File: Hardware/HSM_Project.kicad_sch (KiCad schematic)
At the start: 0 parts

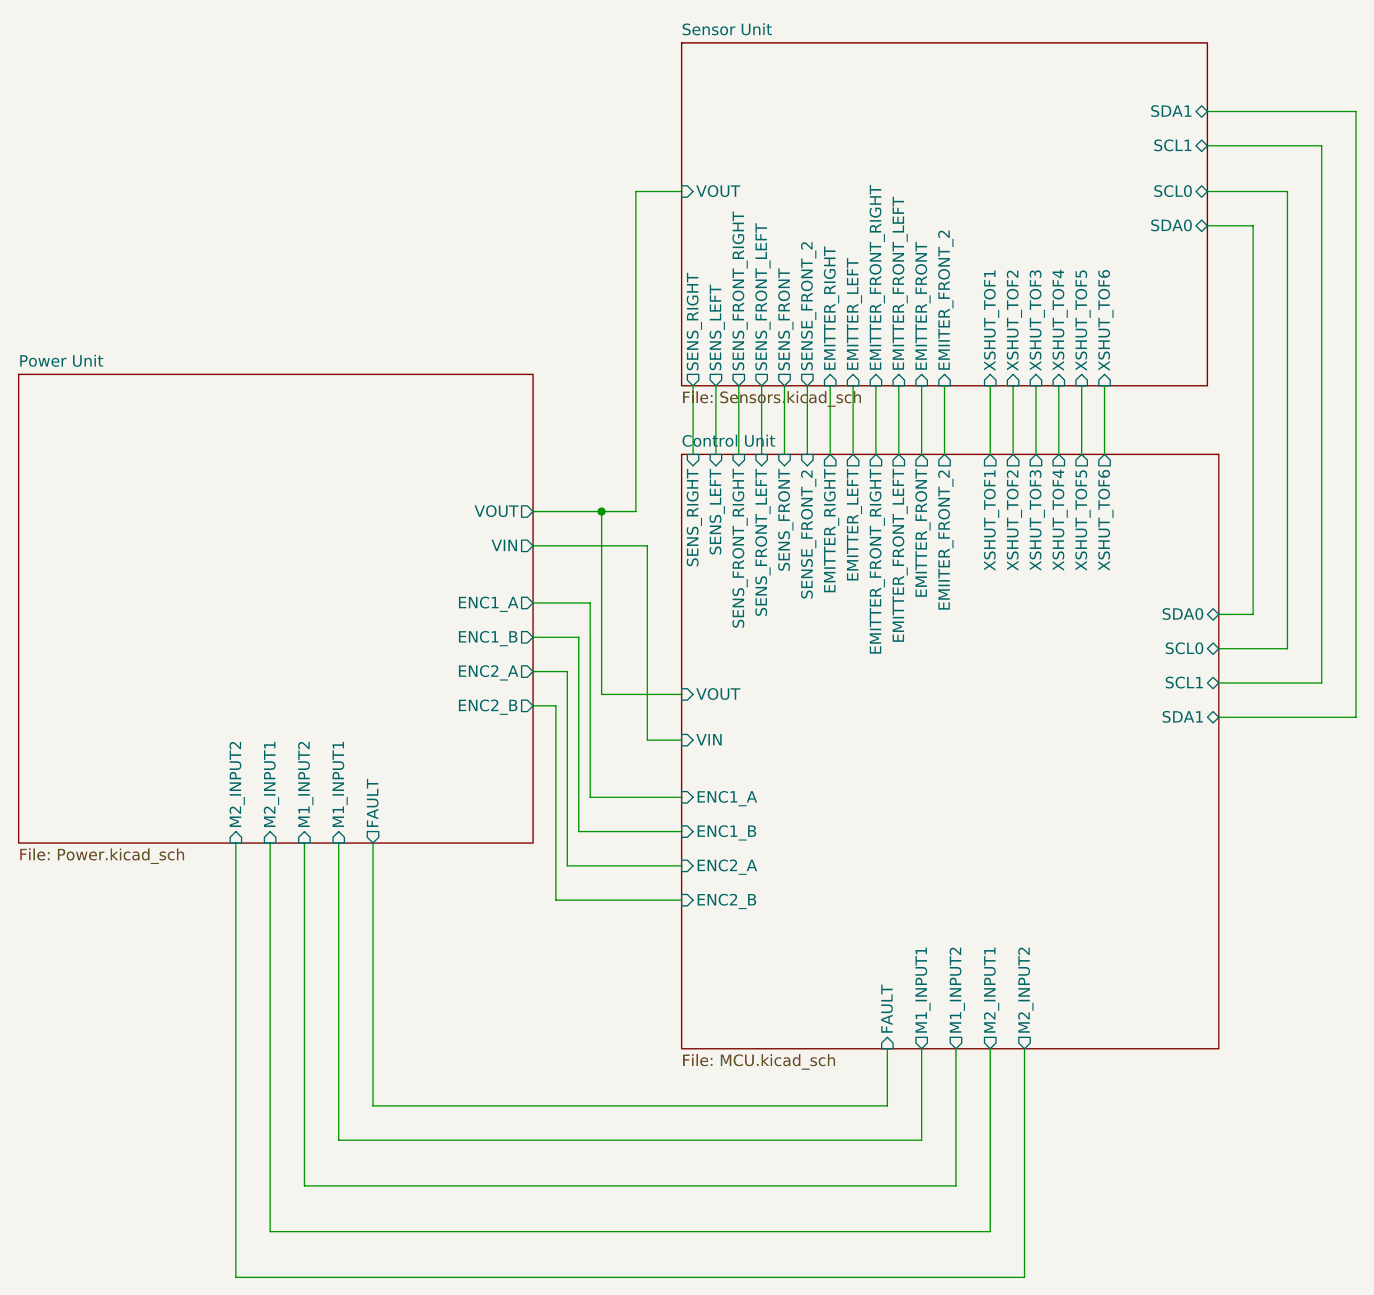
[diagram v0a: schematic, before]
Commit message: Final updated pcb and schematic before dfm check
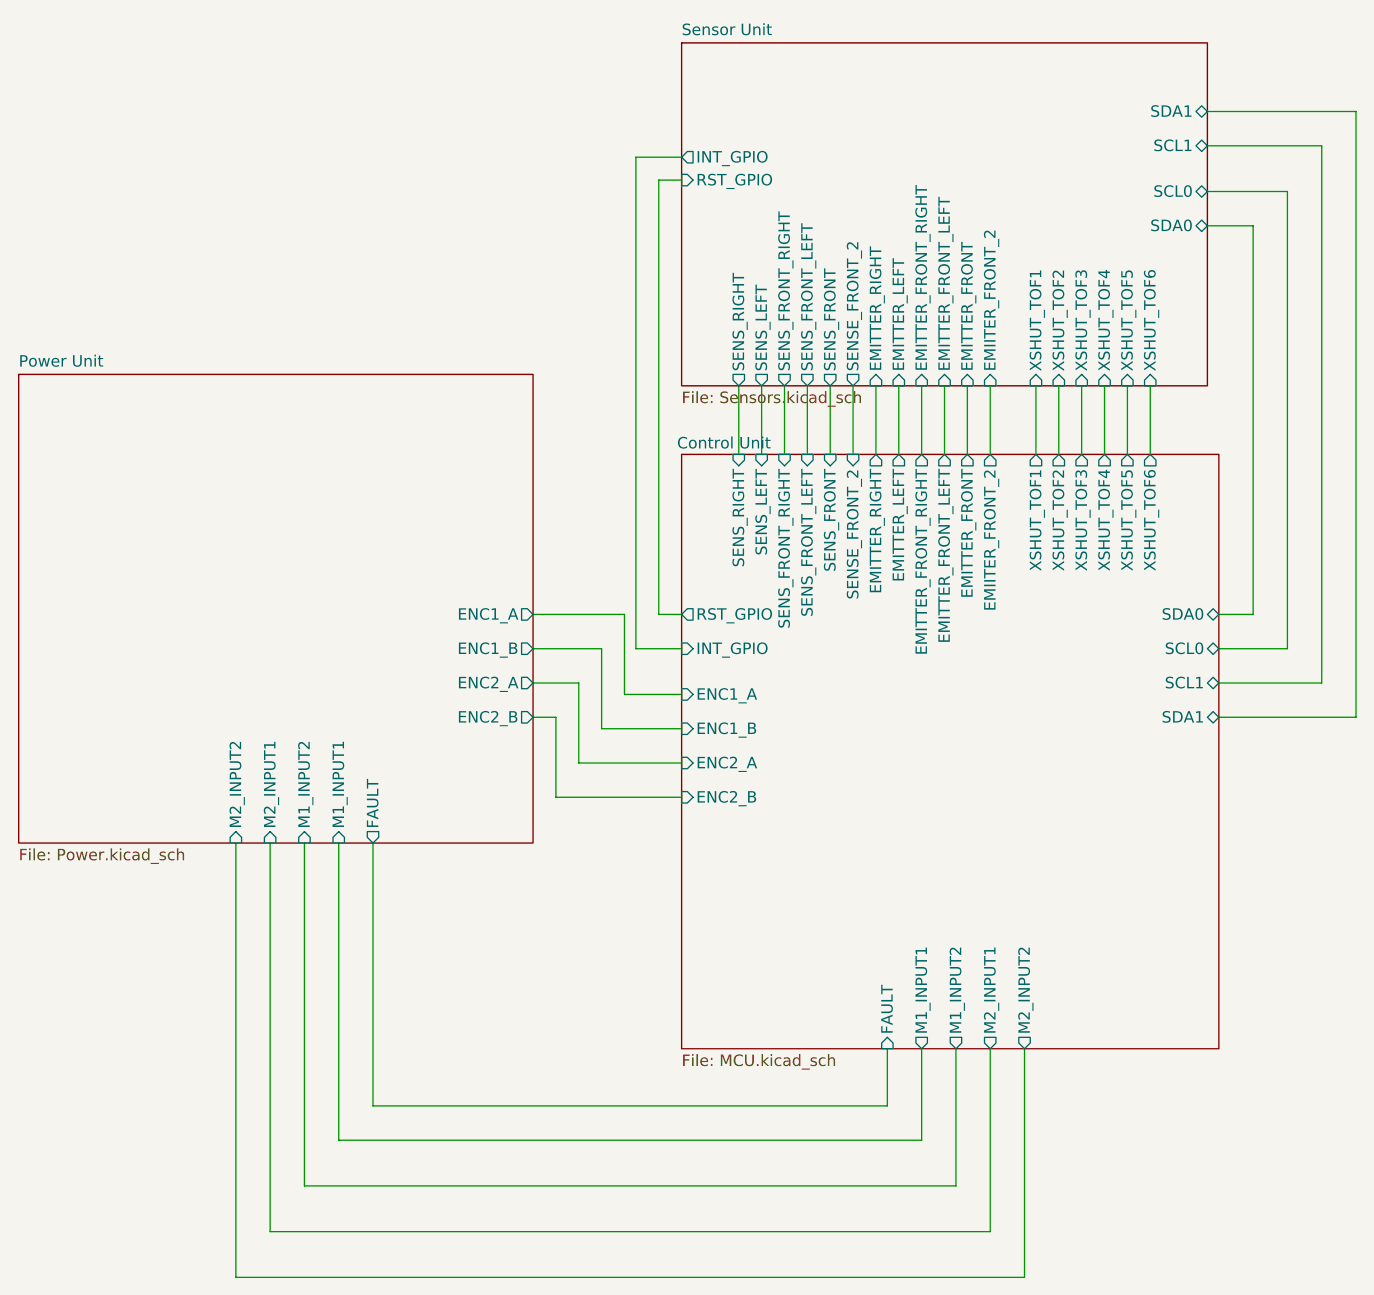
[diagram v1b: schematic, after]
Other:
- sheet Control Unit ports: added INT_GPIO, RST_GPIO; removed VIN, VOUT
- sheet Power Unit ports: added none; removed VIN, VOUT
- sheet Sensor Unit ports: added INT_GPIO, RST_GPIO; removed VOUT
